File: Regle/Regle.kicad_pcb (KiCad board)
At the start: 2 copper layers, 100 x 32 mm, 25 parts

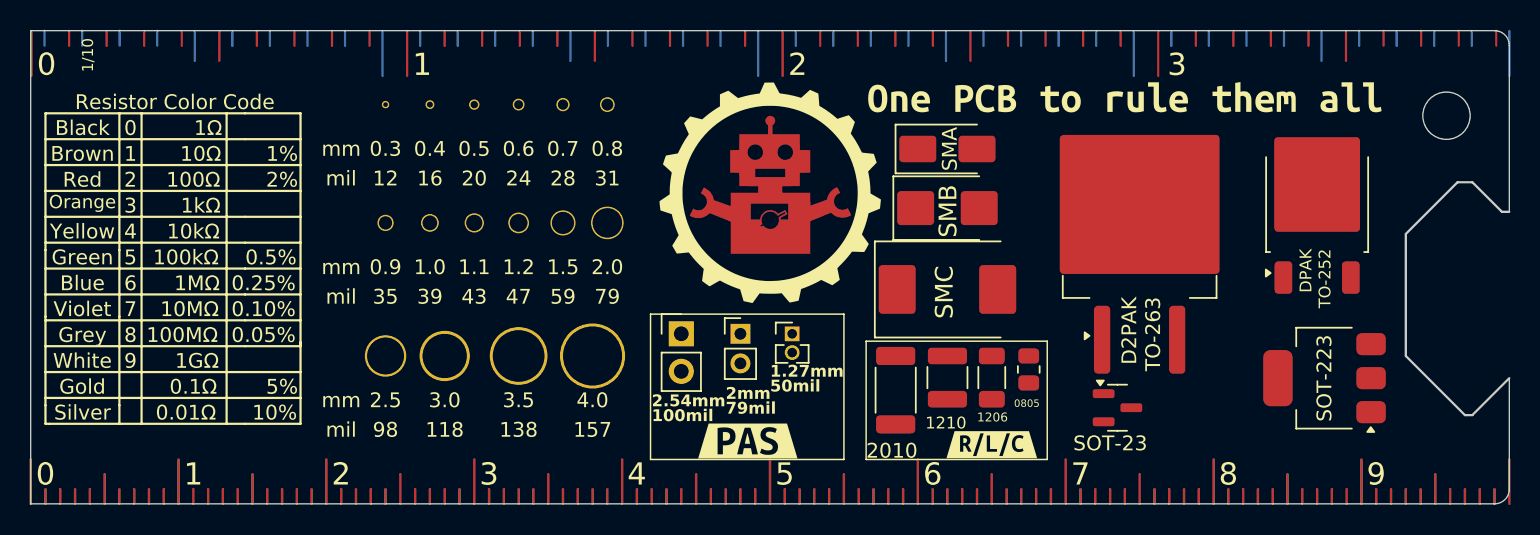
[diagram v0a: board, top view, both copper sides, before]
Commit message: Cartes élec à refaire et TODO
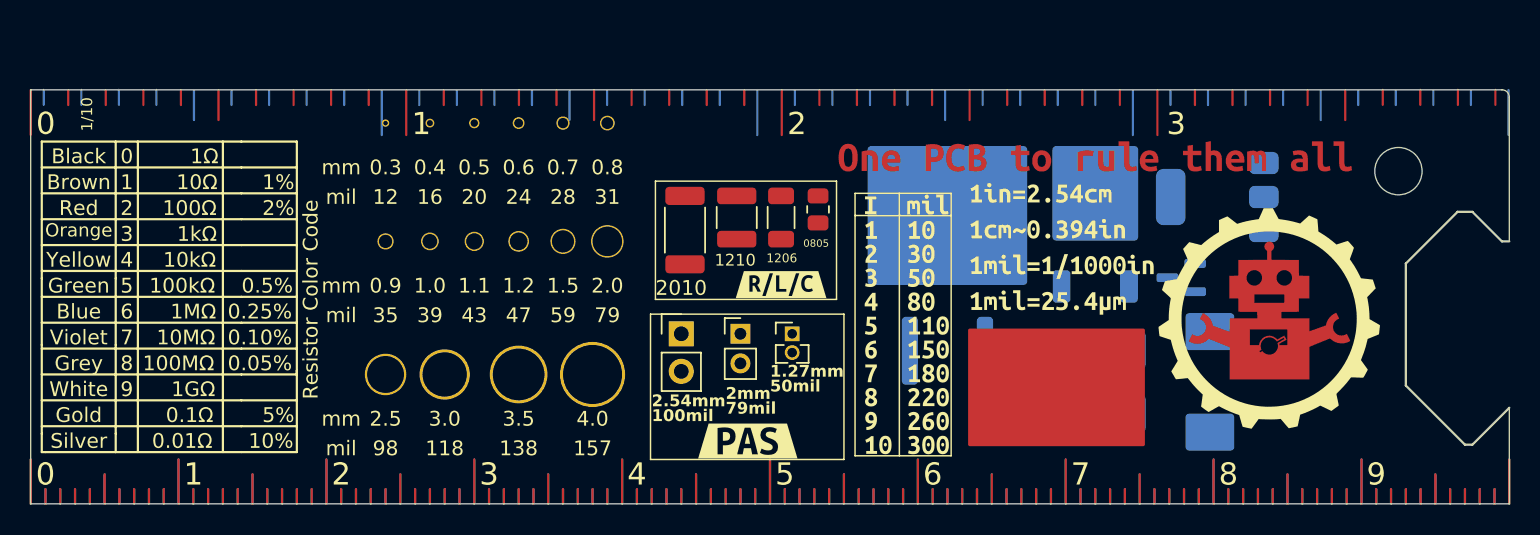
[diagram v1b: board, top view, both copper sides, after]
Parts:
- removed kibuzzard-66C1E3AE: G***, kibuzzard-66C1E3AE
- added kibuzzard-66D03D47: G***, kibuzzard-66D03D47, F.Cu at (211.0, 63.5)
- added kibuzzard-66D03D62: G***, kibuzzard-66D03D62, F.Cu at (211.0, 63.5)
- added kibuzzard-66DA2F2F: G***, kibuzzard-66DA2F2F, F.Cu at (208.8, 69.8)
- added kibuzzard-66DA31A3: G***, kibuzzard-66DA31A3, F.Cu at (198.2, 75.8)
- added kibuzzard-66DA31DF: G***, kibuzzard-66DA31DF, F.Cu at (198.2, 66.8)
- REF** (x7): moved to B.Cu
- moved G*** 34.8 mm to (222.8, 74.5)
- moved REF** 18.8 mm to (218.8, 78.8), turned to -90 degrees
- moved REF** 17.9 mm to (186.8, 67.6)
- moved REF** 17.9 mm to (183.2, 68.5)
- moved REF** 17.9 mm to (189.8, 67.6)
- moved kibuzzard-66C2FC0E 17.9 mm to (189.8, 72.2)
- moved REF** 17.9 mm to (192.2, 67.1)
- moved REF** 17.8 mm to (209.2, 78.8), turned to -90 degrees
- moved REF** 17.0 mm to (213.2, 78.8), turned to -90 degrees
- moved REF** 15.0 mm to (211.0, 67.3)
- moved REF** 14.2 mm to (219.2, 66.2)
- moved REF** 13.0 mm to (201.0, 69.0)
- moved REF** 9.80 mm to (216.8, 71.7), turned to 180 degrees
- moved REF** 4.96 mm to (231.5, 64.5)
- moved REF** 4.00 mm to (238.9, 59.0)
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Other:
- board size 100 x 32 mm -> 100 x 28 mm
- board text added: "SOT-223"
